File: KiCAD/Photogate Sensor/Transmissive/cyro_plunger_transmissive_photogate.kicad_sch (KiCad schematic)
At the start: 32 parts, among them J1 USB_B_Micro, J2 UPDI socket, Q1 Q_NMOS_GSD, U1 Opamp_Dual, U2 CH340C, U3 ATTiny1614, U4 5V LDO, U5 AD5242BRUZ1M

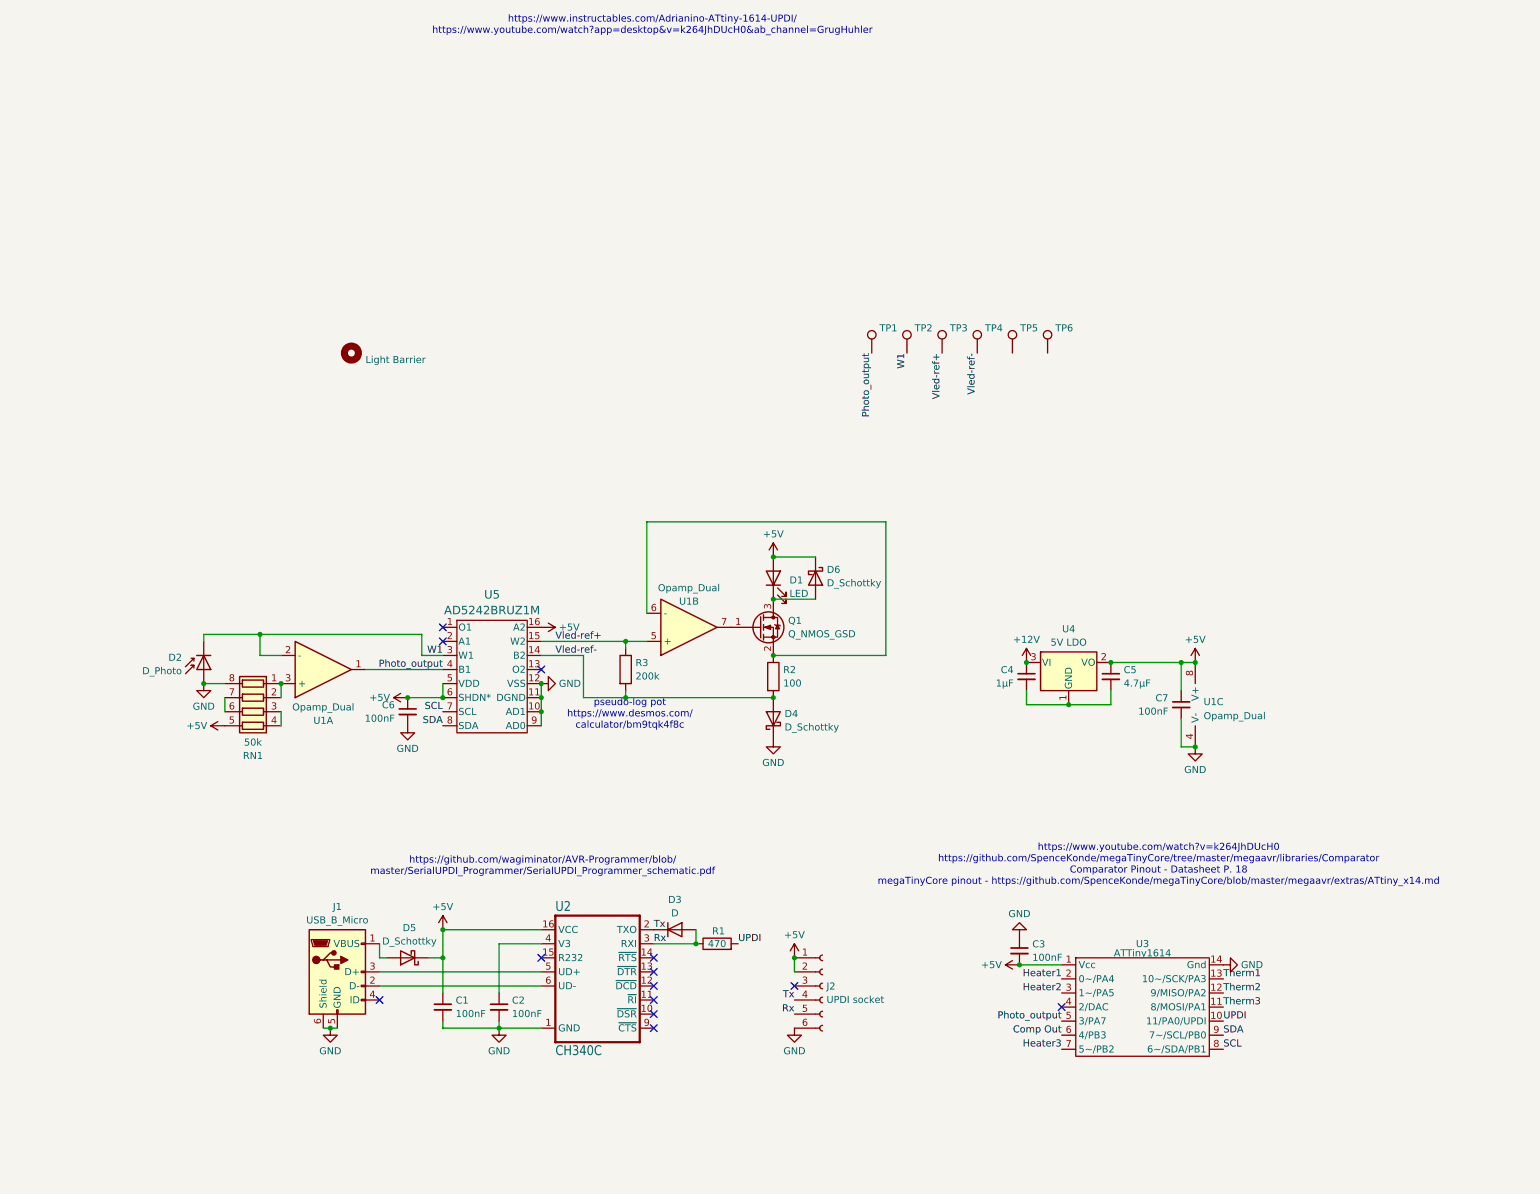
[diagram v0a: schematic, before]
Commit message: Finish draft of schematic, started on board
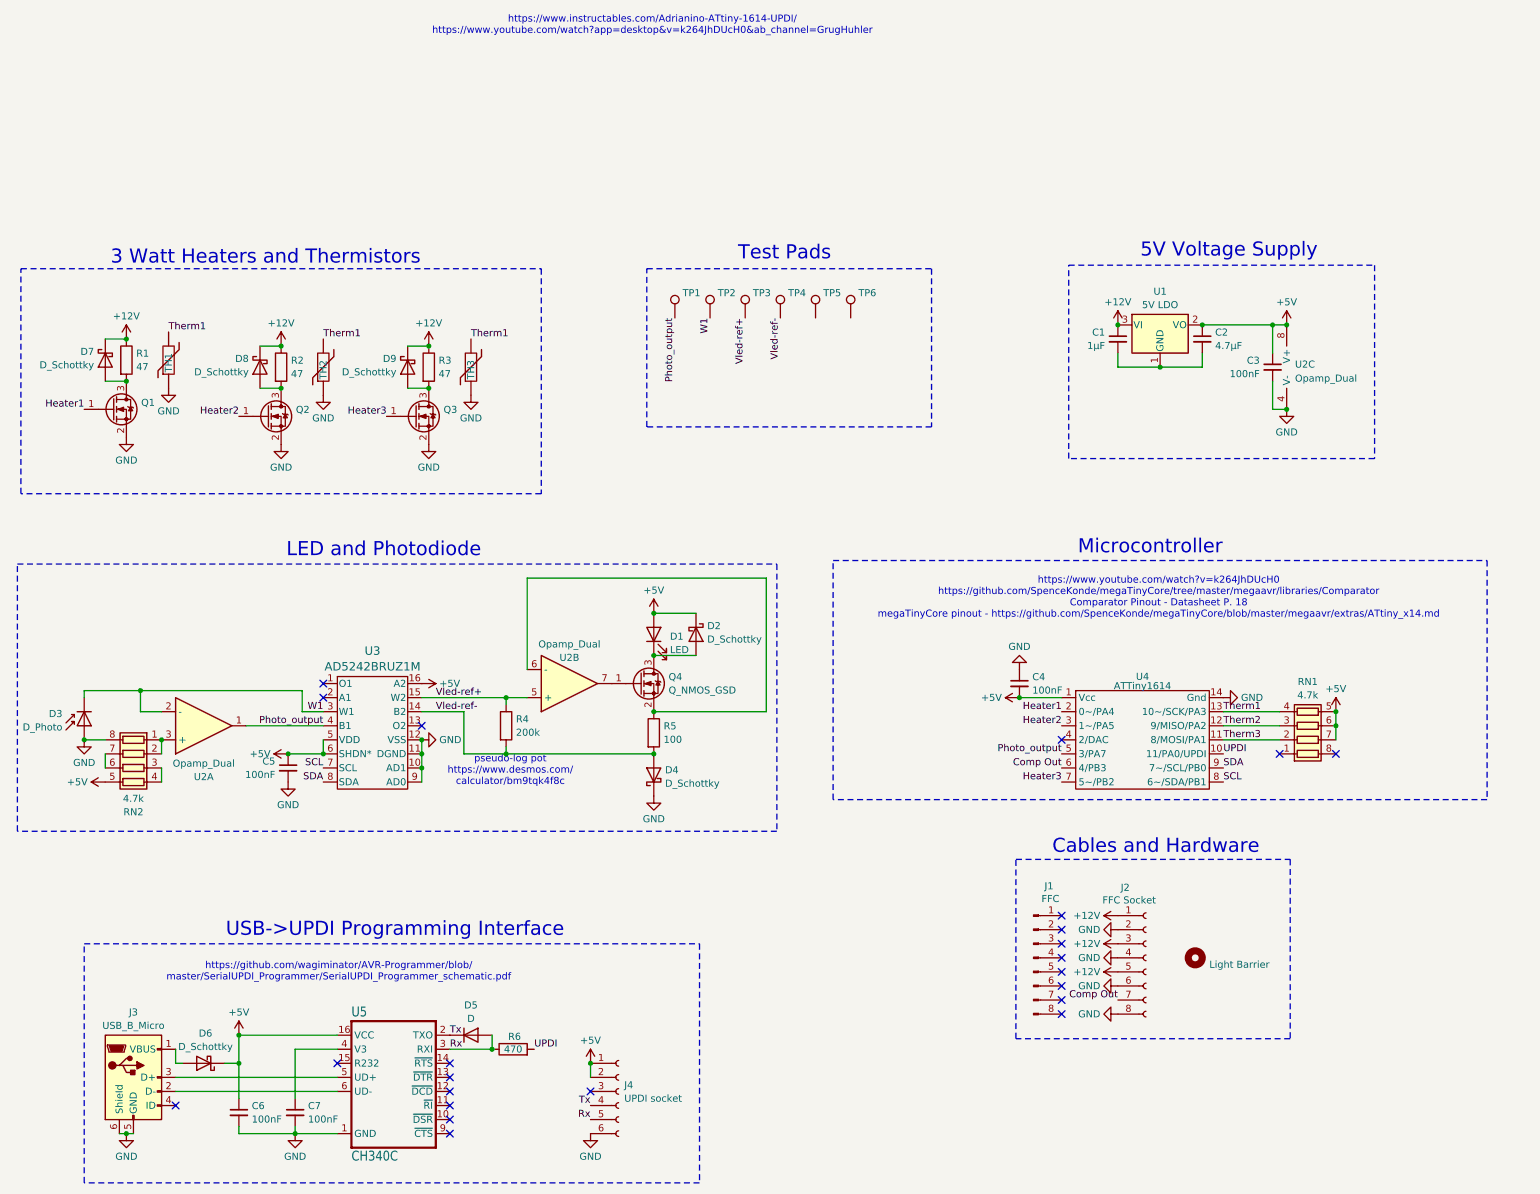
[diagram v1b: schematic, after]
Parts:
- added D7, D8, D9: D_Schottky, Diode_SMD:D_SOD-323, symbol Device:D_Schottky
- added J1: FFC, symbol Connector:Conn_01x08_Pin
- added J2: FFC Socket, Custom:AMPHENOL_SFW8S-2STE1LF, symbol Connector:Conn_01x08_Socket
- added Q1, Q2, Q3: Q_NMOS_GSD, Package_TO_SOT_SMD:SOT-23-3, symbol Device:Q_NMOS_GSD
- added R1, R2, R3: 47, Custom:RES_SMF5_TYCO_TYC, symbol Device:R
- added RN1: 4.7k, Resistor_SMD:R_Array_Convex_4x1206, symbol Device:R_Pack04
- added TH1, TH2, TH3: Thermistor, Resistor_SMD:R_0805_2012Metric, symbol Device:Thermistor
- J3: renamed from J1; footprint Custom:AMPHENOL_10118193-0001LF -> Custom:CUI_UJ2-MIBH-G-SMT-TR; Manufacturer Amphenol ICC (FCI) -> Same Sky (Formerly CUI Devices); Part 10118193-0001LF -> UJ2-MIBH-G-SMT-TR
- RN2: renamed from RN1; value 50k -> 4.7k; footprint Resistor_SMD:R_Array_Convex_4x0603 -> Resistor_SMD:R_Array_Convex_4x1206; Manufacturer Vishay Beyschlag/Draloric/BC Components -> YAGEO; Part ACASA5002S5002P1AT -> YC324-FK-074K7L
- U3: renamed from U5; footprint RU_16_ADI -> Custom:AD5242BRUZ1M
- renumbered C4 to C1, C5 to C2, C7 to C3, C3 to C4, C6 to C5, C1 to C6, C2 to C7, D6 to D2, D2 to D3, D3 to D5, D5 to D6, J2 to J4, Q1 to Q4, R3 to R4, R2 to R5, R1 to R6, U4 to U1, U1 to U2, U3 to U4, U2 to U5
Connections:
- net +12V: now also D7.1 (K), D8.1 (K), D9.1 (K), J2.1 (Pin_1), J2.3 (Pin_3), J2.5 (Pin_5), R1.1, R2.1, R3.1
- net +5V: now also RN1.5 (R4.2), RN1.6 (R3.2), RN1.7 (R2.2)
- net Comp Out: now also J2.7 (Pin_7)
- net GND: now also J2.2 (Pin_2), J2.4 (Pin_4), J2.6 (Pin_6), J2.8 (Pin_8), Q1.2 (S), Q2.2 (S), Q3.2 (S), TH1.1, TH2.1, TH3.1
- net Heater1: now also Q1.1 (G)
- net Heater2: now also Q2.1 (G)
- net Heater3: now also Q3.1 (G)
- net Therm1: now also RN1.4 (R4.1), TH1.2, TH2.2, TH3.2
- net Therm2: now also RN1.3 (R3.1)
- net Therm3: now also RN1.2 (R2.1)
- new net: D8.2 (A), Q2.3 (D), R2.2
- new net: D9.2 (A), Q3.3 (D), R3.2
- new net: D7.2 (A), Q1.3 (D), R1.2
- no-connect marks 13 -> 23
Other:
- note added: "3 Watt Heaters and Thermistors"
- note added: "5V Voltage Supply"
- note added: "Cables and Hardware"
- note added: "LED and Photodiode"
- note added: "Microcontroller"
- note added: "Test Pads"
- note added: "USB->UPDI Programming Interface"
- moved on the sheet: C1, C2, C3, C4, C5, C6, C7, D1, D2, D3, D4, D5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
